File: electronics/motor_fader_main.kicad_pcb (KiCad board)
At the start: 2 copper layers, 59 x 17 mm, 29 parts, among them J1 Conn_01x04_MountingPin, J2 Program, J3 Conn_01x04_MountingPin, U1 ATtiny816-M, U2 DRV8837

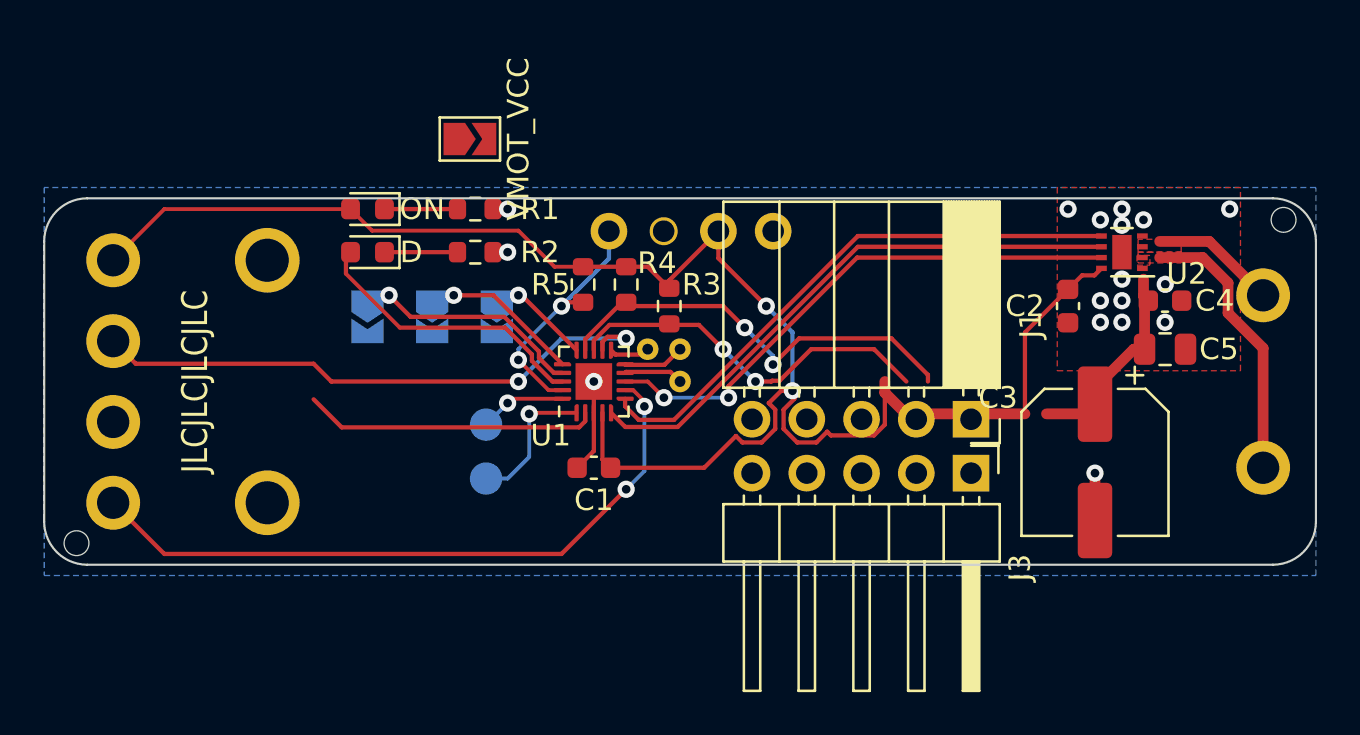
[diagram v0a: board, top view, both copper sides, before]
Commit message: updates
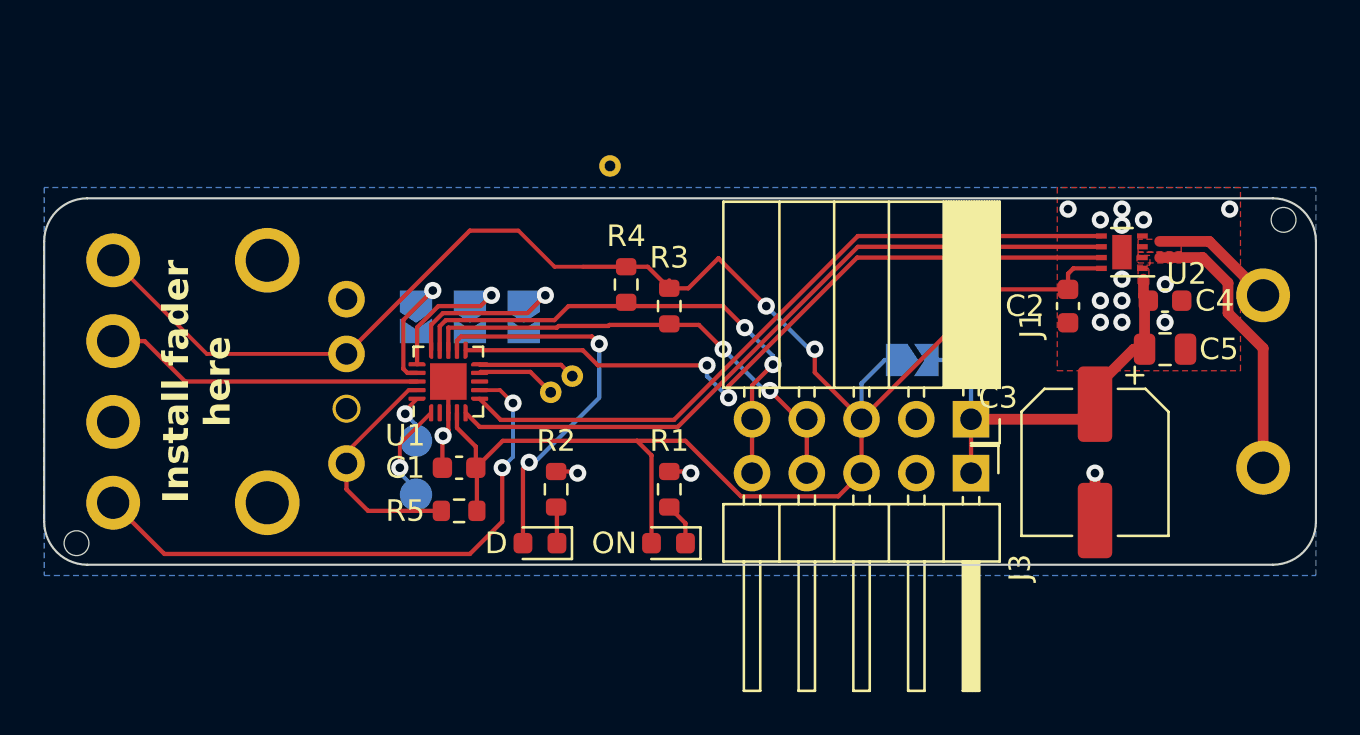
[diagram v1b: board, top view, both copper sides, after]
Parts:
- JP4: moved to B.Cu
- U1: value ATtiny816-M -> ATtiny1616-M
- moved JP4 22.9 mm to (93.3, 49.0)
- moved D1 20.9 mm to (82.0, 57.5)
- moved J2 16.3 mm to (67.0, 53.8), turned to 0 degrees
- moved R1 15.8 mm to (82.0, 55.0), turned to 90 degrees
- moved D2 15.7 mm to (76.0, 57.5)
- moved R5 12.0 mm to (72.2, 56.0), turned to 180 degrees
- moved R2 11.6 mm to (76.8, 55.0), turned to 90 degrees
- moved TP1 8.68 mm to (79.2, 40.0)
- moved U1 6.75 mm to (71.8, 50.0)
- moved C1 6.25 mm to (72.2, 54.0)
- moved TP5 6.02 mm to (76.5, 50.5)
- moved TP4 5.15 mm to (77.5, 49.8)
- moved TP2 3.34 mm to (70.2, 55.2), turned to 180 degrees
- moved TP3 3.34 mm to (70.2, 52.8), turned to 180 degrees
- moved JP3 2.25 mm to (70.2, 47.0)
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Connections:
- U1 pad 12: unconnected-(U1-PB2-Pad12) -> /DBG_LED
- U1 pad 18: /DBG_LED -> /TOUCH
- U1 pad 8: /TOUCH -> unconnected-(U1-PA7-Pad8)
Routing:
- net VCC: track 80.2 -> 95.3 mm
- net unconnected-(U1-PA3-Pad2): track 13.6 -> 0.00 mm
- net /TOUCH: track 27.0 -> 14.9 mm, vias 2 -> 0
- net /V_MOT: track 9.65 -> 19.8 mm
- net /M_1: track 26.5 -> 33.2 mm
- net /M_2: track 26.2 -> 32.8 mm
- net /M_SLEEP: track 27.3 -> 33.7 mm
- net /A0: track 9.72 -> 4.91 mm
- net /DBG_LED: track 13.4 -> 18.1 mm, vias 0 -> 2
- net /SDA: track 17.6 -> 22.0 mm
- net /R_FADER: track 31.6 -> 27.2 mm
- net /SCL: track 19.9 -> 23.8 mm
- net /A2: track 3.76 -> 7.04 mm
- net /RX: track 6.63 -> 4.46 mm
- net Net-(D2-K): track 3.39 -> 1.69 mm
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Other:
- board text added: "Install fader here"
- board text removed: "JLCJLCJLCJLC"

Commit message: Updates
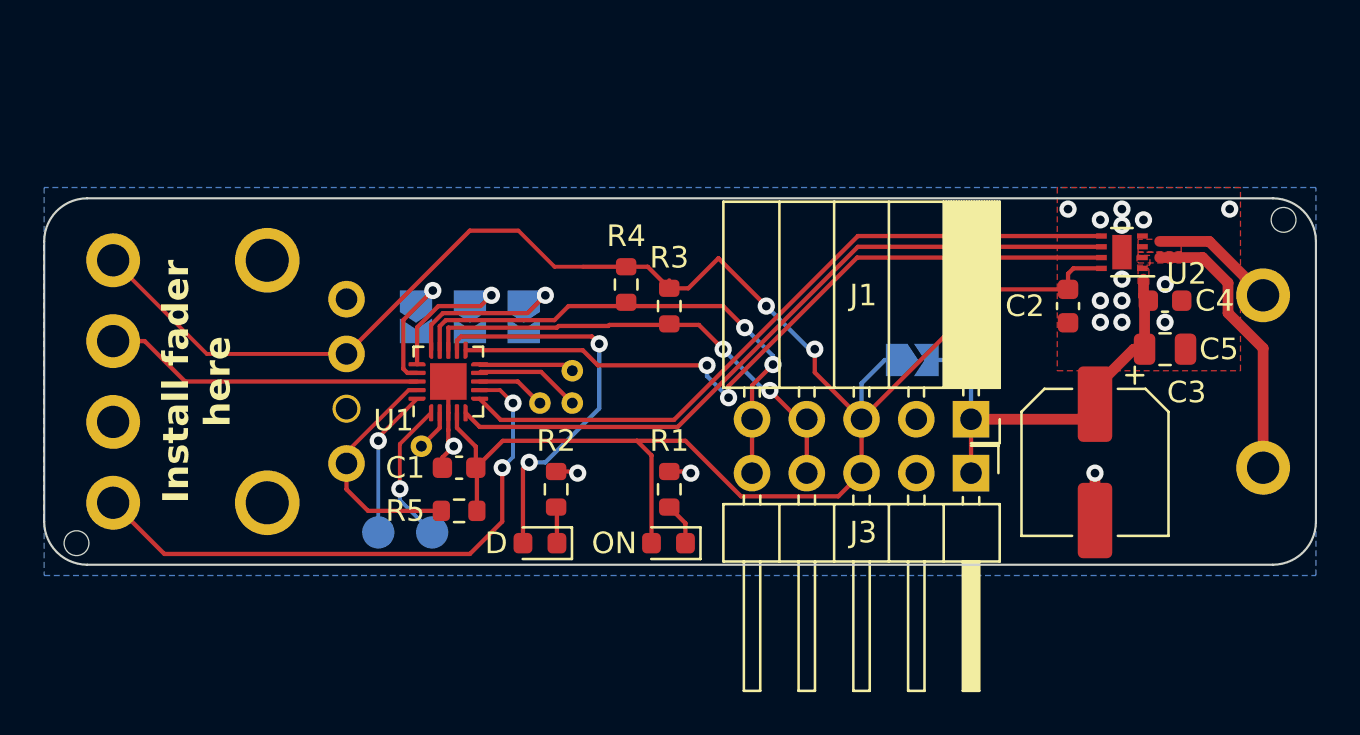
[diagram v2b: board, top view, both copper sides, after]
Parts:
- added TP6: PA3, modified:TestPoint_THTPad_D1.0mm_Drill0.5mm_small_valuesilk, B.Cu at (70.5, 53.0)
- TP1: value P?? -> PA7
- moved TP1 11.5 mm to (76.0, 51.0)
- moved TP3 4.60 mm to (68.5, 57.0)
- moved TP2 1.90 mm to (71.0, 57.0)
- moved TP5 1.12 mm to (77.5, 51.0)
- moved TP4 0.25 mm to (77.5, 49.5)
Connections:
- TP1 pad 1: unconnected-(TP1-Pad1) -> Net-(U1-PA7)
- U1 pad 2: unconnected-(U1-PA3-Pad2) -> Net-(U1-PA3)
- U1 pad 8: unconnected-(U1-PA7-Pad8) -> Net-(U1-PA7)
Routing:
- net /TX: track 2.38 -> 6.95 mm
- net Net-(U1-PA7): track 0.00 -> 3.21 mm
- net /RX: track 4.46 -> 6.77 mm
- net Net-(U1-PA3): track 0.00 -> 1.90 mm
- net Net-(U1-PB5): track 3.71 -> 4.92 mm
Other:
- board text added: "GND"
- board text added: "Motor Fader ${RELEASE_VERSION}"
- board text added: "SCL"
- board text added: "SDA"
- board text added: "VCC"
- board text added: "VMot"
- board text removed: "1U Motor Fader ${RELEASE_VERSION}"

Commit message: minor updates, mostly ready
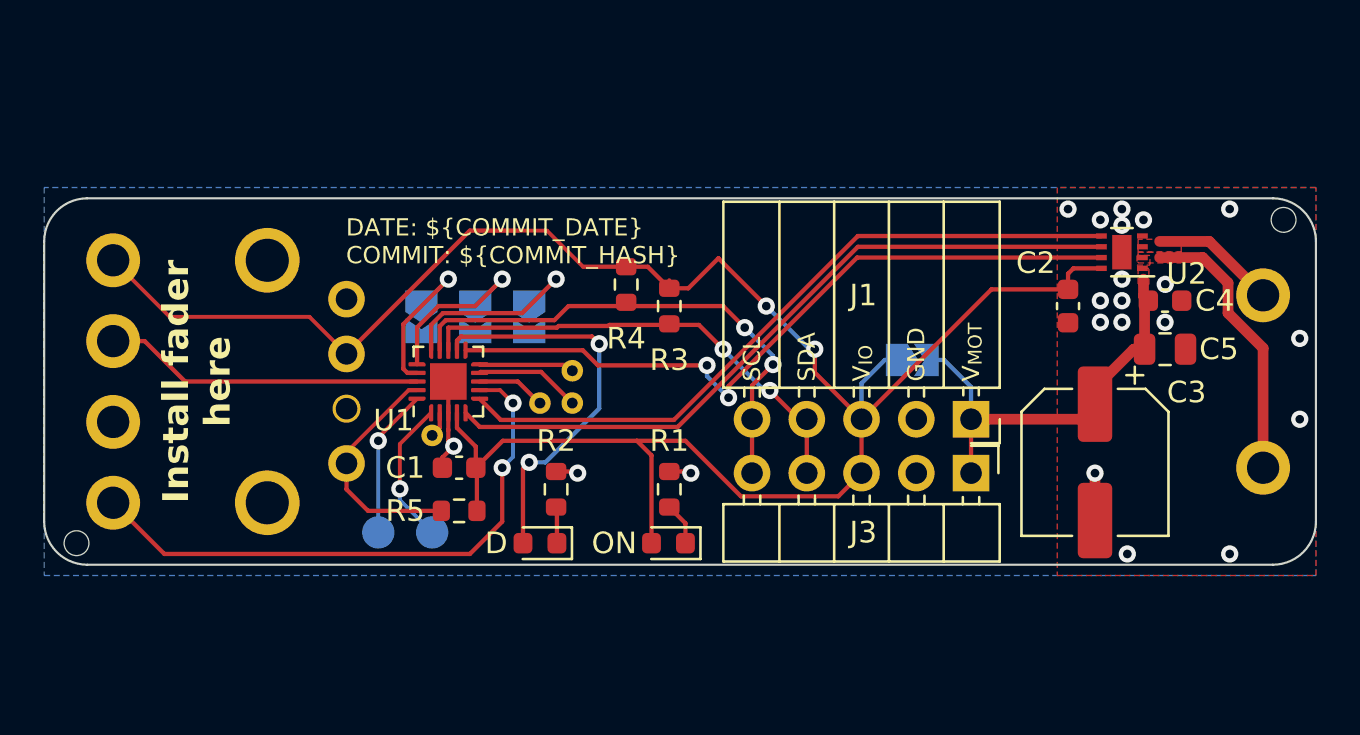
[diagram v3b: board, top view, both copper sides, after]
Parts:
- J1: footprint Connector_PinSocket_2.54mm:PinSocket_1x05_P2.54mm_Horizontal -> modified:PinSocket_1x05_P2.54mm_Horizontal_no_silk_fill
- J3: footprint Connector_PinHeader_2.54mm:PinHeader_1x05_P2.54mm_Horizontal -> modified:PinHeader_1x05_P2.54mm_Horizontal_no_pin_silk
- JP4: value VMOT_VCC -> Vmot <-> Vio; footprint modified:SolderJumper-2_P1.3mm_Open_TrianglePad1.0x1.5mm_thermal_relief -> modified:SolderJumper-2_P1.3mm_Open_TrianglePad1.0x1.5mm_thermal_relief_labelzone
- moved TP6 0.71 mm to (71.0, 52.5)
- moved JP1 0.25 mm to (75.5, 47.0)
- moved JP2 0.25 mm to (73.0, 47.0)
- moved JP3 0.25 mm to (70.5, 47.0)
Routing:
- net /A0: track 4.91 -> 7.42 mm
- net /A1: track 5.78 -> 8.26 mm
- net /A2: track 7.04 -> 9.53 mm
- net Net-(U1-PA3): track 1.90 -> 1.19 mm
- net GND: vias 17 -> 21
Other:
- board text added: "DATE: ${COMMIT_DATE} COMMIT: ${COMMIT_HASH}"
- board text added: "I_{2}C Address"
- board text added: "UPDI"
- board text added: "V_{IO}"
- board text added: "V_{MOT}"
- board text added: "motor fader ${RELEASE_VERSION}"
- board text removed: "DATE: ${COMMIT_DATE_LONG} COMMIT: ${COMMIT_HASH}"
- board text removed: "Motor Fader ${RELEASE_VERSION}"
- board text removed: "VCC"
- board text removed: "VMot"
